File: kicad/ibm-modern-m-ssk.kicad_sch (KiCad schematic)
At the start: 52 parts, among them J1 TF38-24S-0.5SV(830), J2 Molex PicoBlade, J3 Conn_02x06_Odd_Even, J4 Conn_01x04_Pin, J5 726386-2, J6 Conn_Coaxial_Small, Q1 PMZB350UPE,315, SW90 SW_Push, U1 NRF52840, U2 nPM1300-QEAA, Y2 32.768 kHz

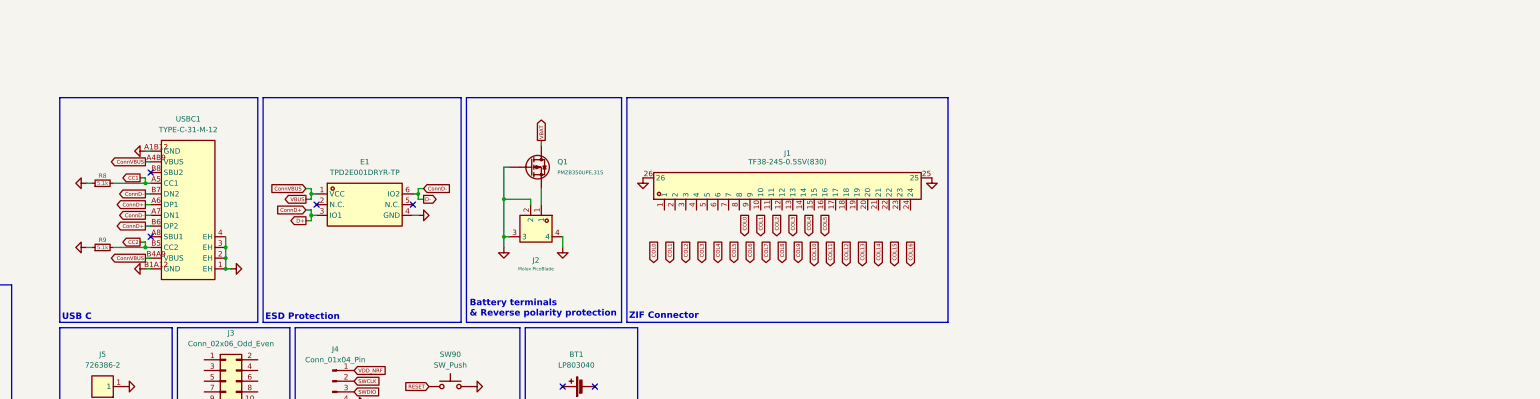
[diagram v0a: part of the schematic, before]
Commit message: update
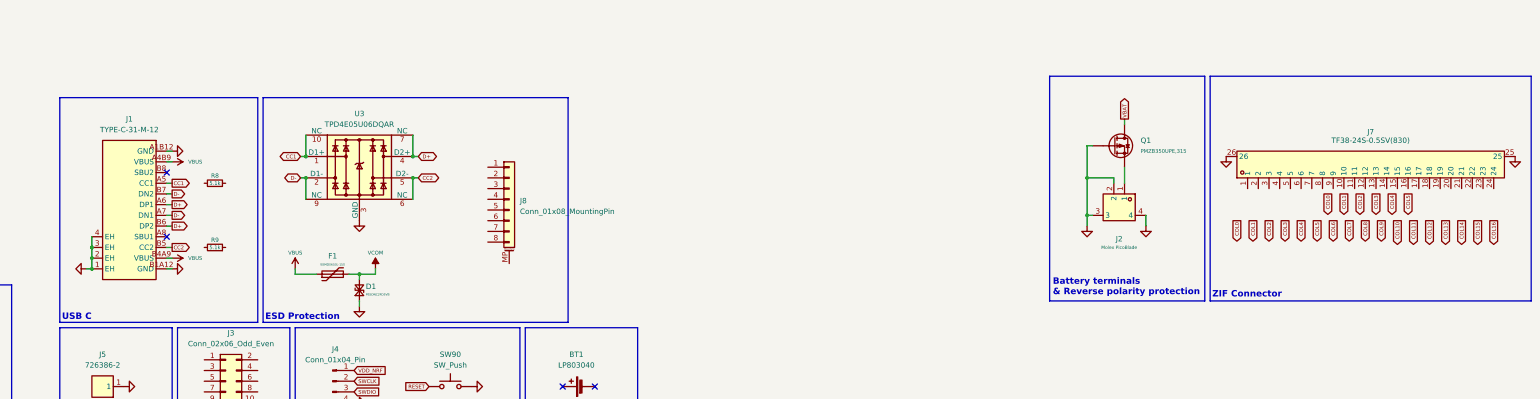
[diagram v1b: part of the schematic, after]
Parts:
- removed E1: TPD2E001DRYR-TP, easyeda2kicad:SON-6_L1.4-W1.0-P0.50-TL_USBULC6-2M6, symbol easyeda2kicad:TPD2E001DRYR-TP
- added D1: PESDNC2FD5VB, easyeda2kicad:Diodes_DFN1006-2, symbol Device:D_TVS_Small
- added F1: BSMD0603L-150, Fuse:Fuse_0603_1608Metric, symbol Device:Polyfuse
- added J8: Conn_01x08_MountingPin, Connector_FFC-FPC:Amphenol_F32Q-1A7x1-11008_1x08-1MP_P0.5mm_Horizontal, symbol Connector_Generic_MountingPin:Conn_01x08_MountingPin
- added U3: TPD4E05U06DQAR, Package_SON:USON-10_2.5x1.0mm_P0.5mm, symbol Power_Protection:TPD4E05U06DQA
- renumbered USBC1 to J1, J1 to J7
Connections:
- net CC1: now also U3.1 (D1+), U3.10 (NC); no longer R8.2
- net CC2: now also U3.5 (D2-), U3.6 (NC); no longer R9.2
- net GND: now also D1.1 (A1), U3.3 (GND), U3.8 (GND); no longer R8.1, R9.1
- net ConnD+ renamed D+
- net D+: now also U3.4 (D2+), U3.7 (NC)
- net ConnD- renamed D-
- net D-: now also U3.2 (D1-), U3.9 (NC)
- net ConnVBUS renamed VBUS
- net VBUS: now also F1.1
- new net VCOM: D1.2 (A2), F1.2
- no-connect marks 15 -> 13
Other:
- moved on the sheet: J1, J2, J7, Q1, R8, R9
